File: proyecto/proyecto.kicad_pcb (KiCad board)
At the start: 2 copper layers, 109 parts, among them J1 Conn_01x03, J2 Conn_01x03, J3 USB_A, J4 Conn_ARM_JTAG_SWD_20, J5 USB_B_Mini, J6 USB_A, J7 Conn_ARM_JTAG_SWD_20, J8 USB_B_Mini, J9 Conn_ARM_JTAG_SWD_20, Q1 Q_PMOS_DSG, Q2 Q_PMOS_DSG, SW1 SW_Push, SW2 SW_Push, SW3 SW_Push, U1 DRV8848, U10 STM32L052C6Tx, U11 LM1117-5.0, U12 LM1117-5.0, U2 Omega2+, U3 MCP73811T-435I-OT, U4 LM1117-3.3, U5 TPS61200DRC, U6 Omega2+, U7 LM1117-3.3, U8 MCP73811T-435I-OT, U9 TPS61200DRC, Y1 24M

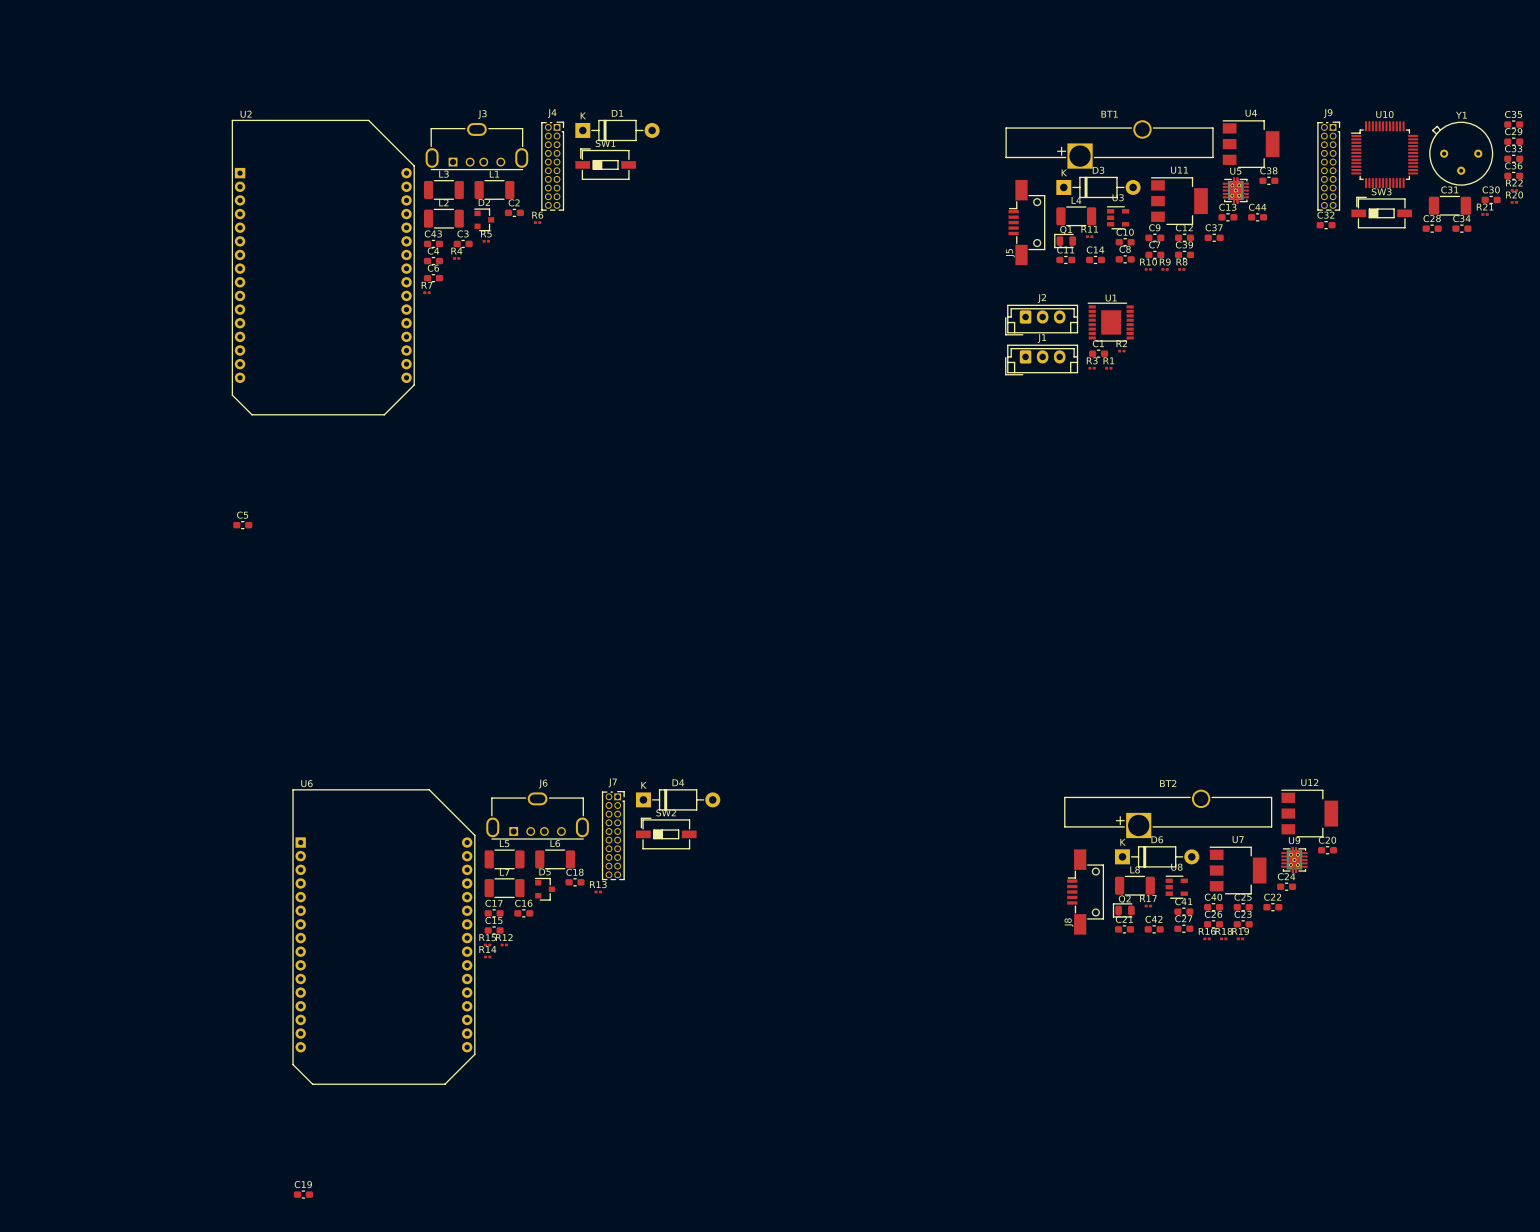
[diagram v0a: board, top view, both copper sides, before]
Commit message: Add files via upload
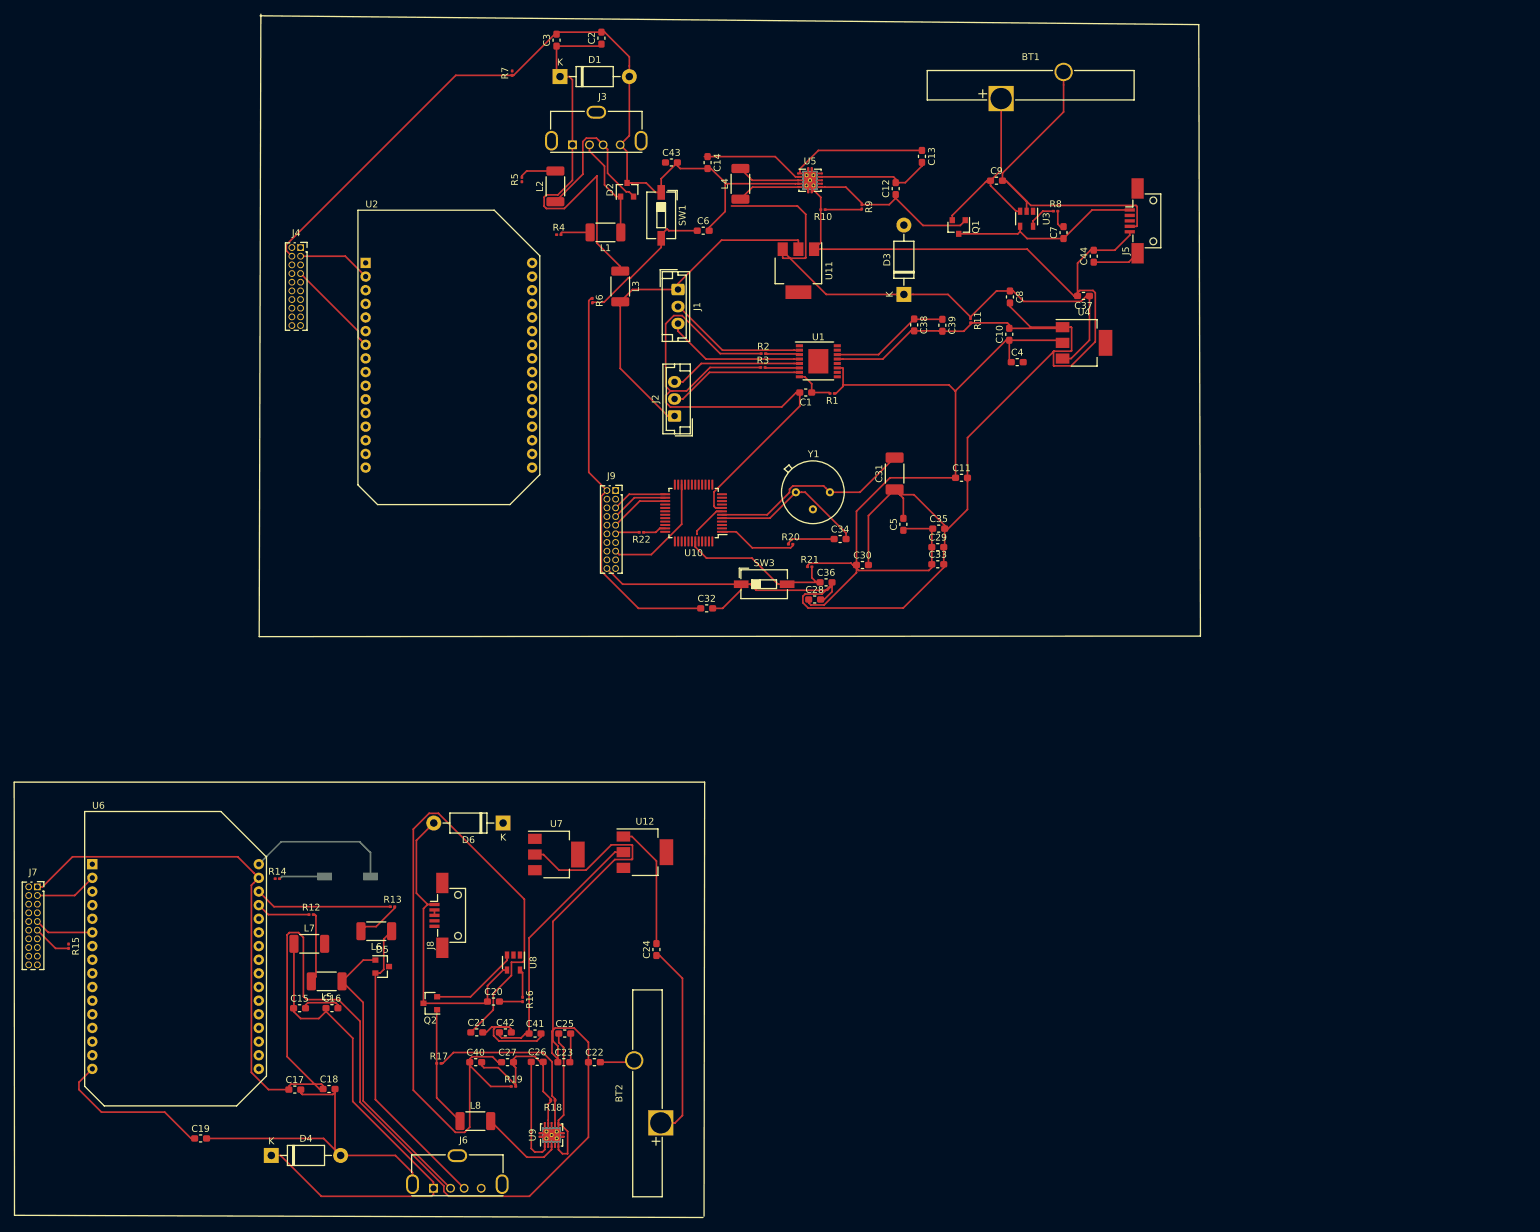
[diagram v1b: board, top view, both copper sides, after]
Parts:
- Q1, Q2: footprint Diode_SMD:D_0805_2012Metric -> Package_TO_SOT_SMD:SOT-23
- SW2: moved to B.Cu
- moved R22 137.4 mm to (113.5, 89.4), turned to 180 degrees
- moved C20 124.3 mm to (91.8, 158.2)
- moved J9 117.9 mm to (109.7, 83.3)
- moved R20 117.3 mm to (135.4, 91.2)
- moved C36 117.1 mm to (140.6, 96.8)
- moved U9 116.1 mm to (100.3, 177.8), turned to 90 degrees
- moved U10 114.1 mm to (121.2, 86.6), turned to 180 degrees
- moved R21 111.7 mm to (138.2, 94.5)
- moved C40 110.5 mm to (89.2, 167.1)
- moved R19 108.7 mm to (94.8, 170.7)
- moved Y1 107.2 mm to (136.1, 83.6)
- moved C32 106.8 mm to (123.1, 100.6)
- moved C30 106.6 mm to (145.9, 94.2)
- moved R17 106.5 mm to (83.8, 167.3)
- moved C28 105.6 mm to (138.9, 99.3)
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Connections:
- U10 pad 25: /Microcontrolador/TCK1 -> /Microcontrolador/TD11
- U10 pad 27: /Microcontrolador/TD01 -> /Microcontrolador/TCK1
- U10 pad 28: /Microcontrolador/TD11 -> /Microcontrolador/TD01
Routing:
- net GND: track 0.00 -> 570.0 mm
- net +3V0: track 0.00 -> 259.1 mm
- net +3V8: track 0.00 -> 180.3 mm
- net GNDA: track 0.00 -> 147.8 mm
- net +5VP: track 0.00 -> 118.1 mm
- net +5VL: track 0.00 -> 101.2 mm
- net Net-(C15-Pad1): track 0.00 -> 75.7 mm
- net +5V: track 0.00 -> 69.8 mm
- net Net-(C2-Pad1): track 0.00 -> 59.8 mm
- net Net-(C20-Pad1): track 0.00 -> 45.0 mm
- net Net-(D5-Pad2): track 0.00 -> 44.5 mm
- net Net-(D5-Pad1): track 0.00 -> 43.1 mm
- net Net-(BT2-Pad1): track 0.00 -> 42.2 mm
- net Net-(C25-Pad1): track 0.00 -> 39.2 mm
- net +5VD: track 0.00 -> 38.3 mm
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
